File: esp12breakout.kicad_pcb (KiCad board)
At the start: 2 copper layers, 90.2 x 66 mm, 11 parts, among them P1 CONN_01X08, P2 CONN_01X08, P3 CONN_01X06, U2 ESP-12E

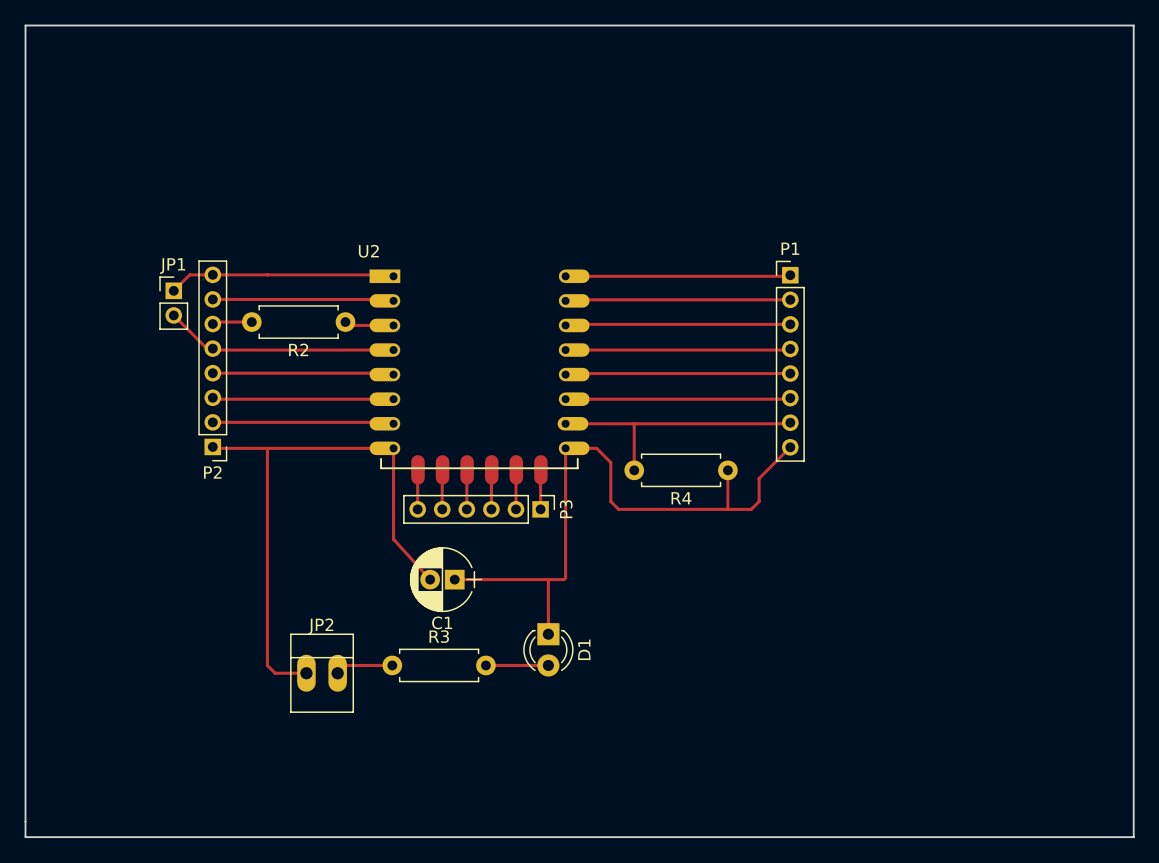
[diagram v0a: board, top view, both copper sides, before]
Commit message: power input en vias
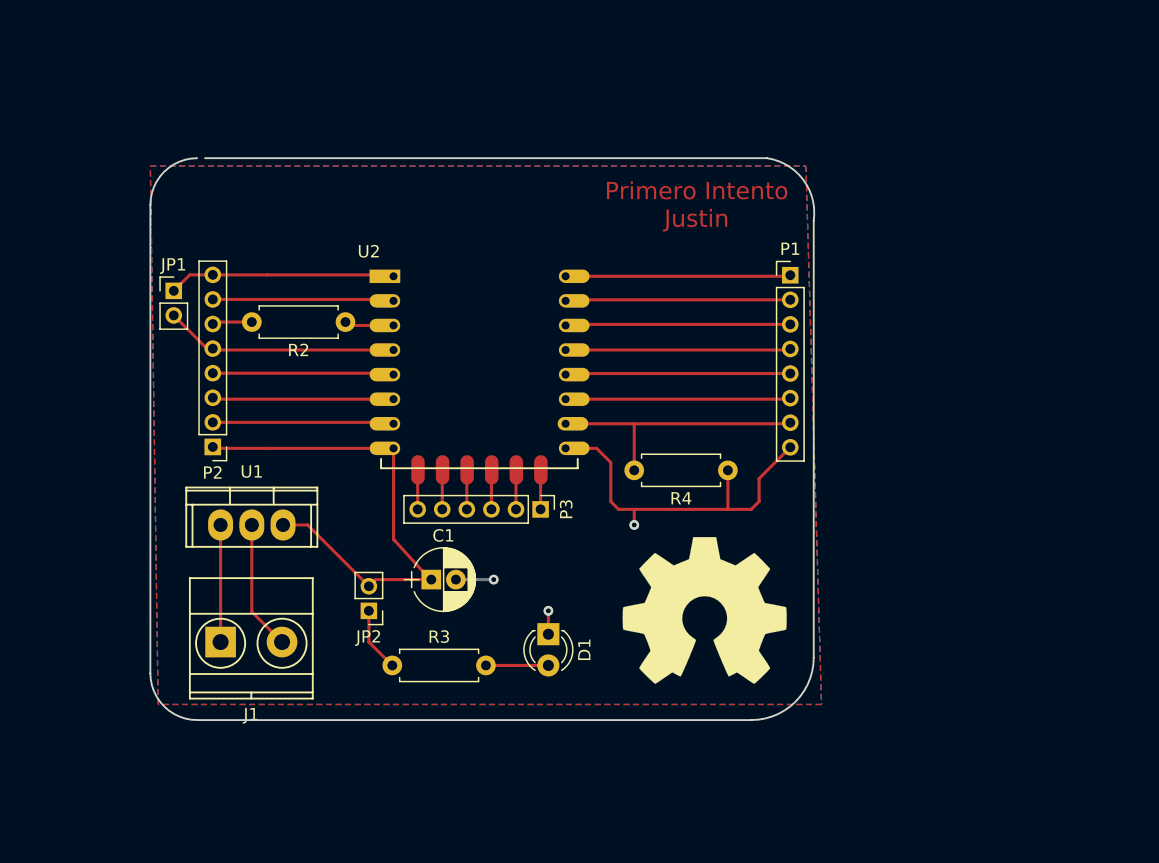
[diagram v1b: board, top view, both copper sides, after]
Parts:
- added J1: Screw_Terminal_1x02, Connectors_Terminal_Blocks:TerminalBlock_Pheonix_MKDS1.5-2pol, F.Cu at (121.3, 81.9)
- added REF***: OSHW-Symbol_13.4x12mm_SilkScreen, Symbols:OSHW-Symbol_13.4x12mm_SilkScreen, F.Cu at (160.7, 79.4)
- added U1: SPX2920U-3.3, Power_Integrations:TO-220, F.Cu at (123.8, 72.4)
- JP2: value Jumper_NO_Small -> Jumper; footprint Connectors:PINHEAD1-2 -> Pin_Headers:Pin_Header_Straight_1x02_Pitch2.00mm
- moved JP2 7.18 mm to (133.3, 79.4), turned to 180 degrees
- moved C1 1.91 mm to (138.4, 76.8), turned to 0 degrees
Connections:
- C1 pad 1: GND -> VCC
- C1 pad 2: VCC -> GND
- JP2 pad 1: VCC -> Net-(JP2-Pad1)
- JP2 pad 2: Net-(JP2-Pad2) -> VCC
- R3 pad 1: Net-(JP2-Pad2) -> Net-(JP2-Pad1)
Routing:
- net Net-(J1-Pad1): track 0.00 -> 9.53 mm
- net GND: track 52.9 -> 45.6 mm, vias 0 -> 3
- net VCC: track 47.7 -> 40.8 mm
- net Net-(JP2-Pad1): track 0.00 -> 5.23 mm
- net Net-(JP2-Pad2): track 4.71 -> 0.00 mm
- added copper zone on B.Cu, net GND
- added copper zone on F.Cu, net VCC
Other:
- board size 90.2 x 66 mm -> 54 x 45.7 mm
- board text added: "Primero Intento Justin"
